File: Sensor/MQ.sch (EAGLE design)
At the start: 4 parts

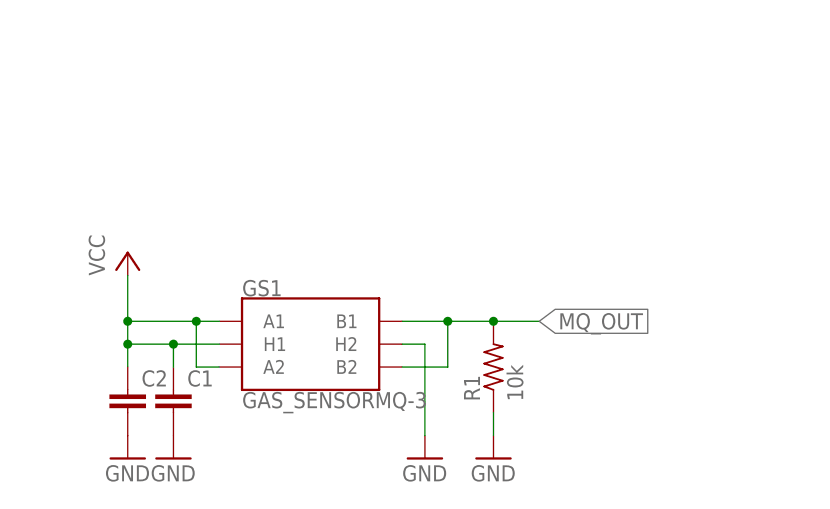
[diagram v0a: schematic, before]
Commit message: Update MQ.sch
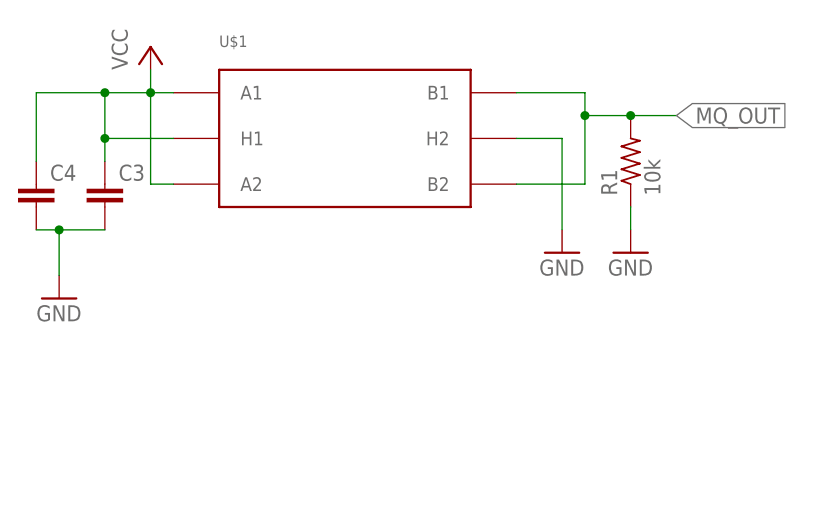
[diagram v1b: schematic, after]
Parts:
- removed C1, C2: (no value), rcl:C-EUC0603
- removed GS1: GAS_SENSORMQ-3, SparkFun-Sensors:GAS_SENSORMQ-3
- added C3, C4: (no value), rcl:C-EUC0603
- added U$1: MQ_GAS_SENSOR_SOCKET, gas_sensor_socket_mq_V2:MQ_GAS_SENSOR_SOCKET
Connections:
- net GND: now also C3.2, C4.2, U$1.H2; no longer C1.2, C2.2, GS1.H2
- net MQ_OUT: now also U$1.B1, U$1.B2; no longer GS1.B1, GS1.B2
- net VCC: now also C3.1, C4.1, U$1.A1, U$1.A2, U$1.H1; no longer C1.1, C2.1, GS1.A1, GS1.A2, GS1.H1
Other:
- moved on the sheet: R1
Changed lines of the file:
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@@
 </classes>
 <parts>
-<part name="P+1" library="supply1" deviceset="VCC" device=""/>
+<part name="U$1" library="gas_sensor_socket_mq_V2" deviceset="MQ_GAS_SENSOR_SOCKET" device=""/>
 <part name="GND1" library="supply1@1" deviceset="GND" device=""/>
 <part name="R1" library="rcl" deviceset="R-US_" device="R0603" value="10k"/>
 <part name="GND2" library="supply1@1" deviceset="GND" device=""/>
-<part name="C1" library="rcl" deviceset="C-EU" device="C0603"/>
-<part name="C2" library="rcl" deviceset="C-EU" device="C0603"/>
-<part name="GND3" library="supply1@1" deviceset="GND" device=""/>
-<part name="GND4" library="supply1@1" deviceset="GND" device=""/>
-<part name="GS1" library="SparkFun-Sensors" deviceset="GAS_SENSOR" device="MQ-3"/>
+<part name="P+2" library="supply1" deviceset="VCC" device=""/>
+<part name="C3" library="rcl" deviceset="C-EU" device="C0603"/>
+<part name="C4" library="rcl" deviceset="C-EU" device="C0603"/>
+<part name="GND5" library="supply1@1" deviceset="GND" device=""/>
 </parts>
 <sheets>
@@
 </plain>
 <instances>
-<instance part="P+1" gate="VCC" x="-5.08" y="88.9" smashed="yes">
-<attribute name="VALUE" x="-7.62" y="86.36" size="1.778" layer="96" rot="R90"/>
+<instance part="U$1" gate="G$1" x="48.26" y="93.98" smashed="yes">
+<attribute name="NAME" x="5.08" y="111.76" size="1.27" layer="95"/>
 </instance>
-<instance part="GND1" gate="1" x="27.94" y="66.04" smashed="yes">
-<attribute name="VALUE" x="25.4" y="63.5" size="1.778" layer="96"/>
+<instance part="GND1" gate="1" x="43.18" y="88.9" smashed="yes">
+<attribute name="VALUE" x="40.64" y="86.36" size="1.778" layer="96"/>
 </instance>
-<instance part="R1" gate="G$1" x="35.56" y="76.2" smashed="yes" rot="R90">
-<attribute name="NAME" x="34.0614" y="72.39" size="1.778" layer="95" rot="R90"/>
-<attribute name="VALUE" x="38.862" y="72.39" size="1.778" layer="96" rot="R90"/>
+<instance part="R1" gate="G$1" x="50.8" y="99.06" smashed="yes" rot="R90">
+<attribute name="NAME" x="49.3014" y="95.25" size="1.778" layer="95" rot="R90"/>
+<attribute name="VALUE" x="54.102" y="95.25" size="1.778" layer="96" rot="R90"/>
 </instance>
-<instance part="GND2" gate="1" x="35.56" y="66.04" smashed="yes">
-<attribute name="VALUE" x="33.02" y="63.5" size="1.778" layer="96"/>
+<instance part="GND2" gate="1" x="50.8" y="88.9" smashed="yes">
+<attribute name="VALUE" x="48.26" y="86.36" size="1.778" layer="96"/>
 </instance>
-<instance part="C1" gate="G$1" x="0" y="73.66" smashed="yes">
-<attribute name="NAME" x="1.524" y="74.041" size="1.778" layer="95"/>
-<attribute name="VALUE" x="1.524" y="68.961" size="1.778" layer="96"/>
+<instance part="P+2" gate="VCC" x="-2.54" y="111.76" smashed="yes">
+<attribute name="VALUE" x="-5.08" y="109.22" size="1.778" layer="96" rot="R90"/>
 </instance>
-<instance part="C2" gate="G$1" x="-5.08" y="73.66" smashed="yes">
-<attribute name="NAME" x="-3.556" y="74.041" size="1.778" layer="95"/>
-<attribute name="VALUE" x="-3.556" y="68.961" size="1.778" layer="96"/>
+<instance part="C3" gate="G$1" x="-7.62" y="96.52" smashed="yes">
+<attribute name="NAME" x="-6.096" y="96.901" size="1.778" layer="95"/>
+<attribute name="VALUE" x="-6.096" y="91.821" size="1.778" layer="96"/>
 </instance>
-<instance part="GND3" gate="1" x="-5.08" y="66.04" smashed="yes">
-<attribute name="VALUE" x="-7.62" y="63.5" size="1.778" layer="96"/>
+<instance part="C4" gate="G$1" x="-15.24" y="96.52" smashed="yes">
+<attribute name="NAME" x="-13.716" y="96.901" size="1.778" layer="95"/>
+<attribute name="VALUE" x="-13.716" y="91.821" size="1.778" layer="96"/>
 </instance>
-<instance part="GND4" gate="1" x="0" y="66.04" smashed="yes">
-<attribute name="VALUE" x="-2.54" y="63.5" size="1.778" layer="96"/>
-</instance>
-<instance part="GS1" gate="G$1" x="15.24" y="78.74" smashed="yes">
-<attribute name="NAME" x="7.62" y="84.074" size="1.778" layer="95" font="vector"/>
-<attribute name="VALUE" x="7.62" y="73.406" size="1.778" layer="96" font="vector" align="top-left"/>
+<instance part="GND5" gate="1" x="-12.7" y="83.82" smashed="yes">
+<attribute name="VALUE" x="-15.24" y="81.28" size="1.778" layer="96"/>
 </instance>
 </instances>
@@
 <net name="VCC" class="0">
 <segment>
-<wire x1="5.08" y1="78.74" x2="0" y2="78.74" width="0.1524" layer="91"/>
-<wire x1="0" y1="78.74" x2="-5.08" y2="78.74" width="0.1524" layer="91"/>
-<wire x1="-5.08" y1="78.74" x2="-5.08" y2="81.28" width="0.1524" layer="91"/>
-<wire x1="-5.08" y1="81.28" x2="2.54" y2="81.28" width="0.1524" layer="91"/>
-<pinref part="P+1" gate="VCC" pin="VCC"/>
-<wire x1="2.54" y1="81.28" x2="5.08" y2="81.28" width="0.1524" layer="91"/>
-<wire x1="-5.08" y1="86.36" x2="-5.08" y2="81.28" width="0.1524" layer="91"/>
-<junction x="-5.08" y="81.28"/>
-<pinref part="C2" gate="G$1" pin="1"/>
-<wire x1="-5.08" y1="76.2" x2="-5.08" y2="78.74" width="0.1524" layer="91"/>
-<junction x="-5.08" y="78.74"/>
-<pinref part="C1" gate="G$1" pin="1"/>
-<wire x1="0" y1="76.2" x2="0" y2="78.74" width="0.1524" layer="91"/>
-<junction x="0" y="78.74"/>
-<pinref part="GS1" gate="G$1" pin="A1"/>
-<pinref part="GS1" gate="G$1" pin="H1"/>
-<pinref part="GS1" gate="G$1" pin="A2"/>
-<wire x1="5.08" y1="76.2" x2="2.54" y2="76.2" width="0.1524" layer="91"/>
-<wire x1="2.54" y1="76.2" x2="2.54" y2="81.28" width="0.1524" layer="91"/>
-<junction x="2.54" y="81.28"/>
+<pinref part="U$1" gate="G$1" pin="A2"/>
+<wire x1="0" y1="96.52" x2="-2.54" y2="96.52" width="0.1524" layer="91"/>
+<wire x1="-2.54" y1="96.52" x2="-2.54" y2="106.68" width="0.1524" layer="91"/>
+<pinref part="U$1" gate="G$1" pin="A1"/>
+<wire x1="-2.54" y1="106.68" x2="0" y2="106.68" width="0.1524" layer="91"/>
+<pinref part="P+2" gate="VCC" pin="VCC"/>
+<wire x1="-2.54" y1="109.22" x2="-2.54" y2="106.68" width="0.1524" layer="91"/>
+<junction x="-2.54" y="106.68"/>
+<wire x1="-2.54" y1="106.68" x2="-7.62" y2="106.68" width="0.1524" layer="91"/>
+<pinref part="C4" gate="G$1" pin="1"/>
+<wire x1="-7.62" y1="106.68" x2="-15.24" y2="106.68" width="0.1524" layer="91"/>
+<wire x1="-15.24" y1="106.68" x2="-15.24" y2="99.06" width="0.1524" layer="91"/>
+<pinref part="C3" gate="G$1" pin="1"/>
+<wire x1="-7.62" y1="99.06" x2="-7.62" y2="101.6" width="0.1524" layer="91"/>
+<junction x="-7.62" y="106.68"/>
+<pinref part="U$1" gate="G$1" pin="H1"/>
+<wire x1="-7.62" y1="101.6" x2="-7.62" y2="106.68" width="0.1524" layer="91"/>
+<wire x1="0" y1="101.6" x2="-7.62" y2="101.6" width="0.1524" layer="91"/>
+<junction x="-7.62" y="101.6"/>
 </segment>
 </net>
 <net name="GND" class="0">
 <segment>
+<wire x1="43.18" y1="91.44" x2="43.18" y2="101.6" width="0.1524" layer="91"/>
 <pinref part="GND1" gate="1" pin="GND"/>
-<wire x1="27.94" y1="68.58" x2="27.94" y2="78.74" width="0.1524" layer="91"/>
-<wire x1="27.94" y1="78.74" x2="25.4" y2="78.74" width="0.1524" layer="91"/>
-<pinref part="GS1" gate="G$1" pin="H2"/>
+<pinref part="U$1" gate="G$1" pin="H2"/>
+<wire x1="38.1" y1="101.6" x2="43.18" y2="101.6" width="0.1524" layer="91"/>
 </segment>
 <segment>
+<wire x1="50.8" y1="93.98" x2="50.8" y2="91.44" width="0.1524" layer="91"/>
 <pinref part="R1" gate="G$1" pin="1"/>
 <pinref part="GND2" gate="1" pin="GND"/>
-<wire x1="35.56" y1="71.12" x2="35.56" y2="68.58" width="0.1524" layer="91"/>
 </segment>
 <segment>
-<pinref part="C2" gate="G$1" pin="2"/>
-<pinref part="GND3" gate="1" pin="GND"/>
-</segment>
-<segment>
-<pinref part="C1" gate="G$1" pin="2"/>
-<pinref part="GND4" gate="1" pin="GND"/>
+<pinref part="C3" gate="G$1" pin="2"/>
+<pinref part="C4" gate="G$1" pin="2"/>
+<wire x1="-7.62" y1="91.44" x2="-12.7" y2="91.44" width="0.1524" layer="91"/>
+<pinref part="GND5" gate="1" pin="GND"/>
+<wire x1="-12.7" y1="91.44" x2="-15.24" y2="91.44" width="0.1524" layer="91"/>
+<wire x1="-12.7" y1="86.36" x2="-12.7" y2="91.44" width="0.1524" layer="91"/>
+<junction x="-12.7" y="91.44"/>
 </segment>
 </net>
 <net name="MQ_OUT" class="0">
 <segment>
+<wire x1="45.72" y1="104.14" x2="50.8" y2="104.14" width="0.1524" layer="91"/>
+<wire x1="50.8" y1="104.14" x2="55.88" y2="104.14" width="0.1524" layer="91"/>
+<junction x="50.8" y="104.14"/>
+<label x="55.88" y="104.14" size="1.778" layer="95" xref="yes"/>
+<wire x1="45.72" y1="96.52" x2="45.72" y2="104.14" width="0.1524" layer="91"/>
+<junction x="45.72" y="104.14"/>
 <pinref part="R1" gate="G$1" pin="2"/>
-<wire x1="25.4" y1="81.28" x2="30.48" y2="81.28" width="0.1524" layer="91"/>
-<wire x1="30.48" y1="81.28" x2="35.56" y2="81.28" width="0.1524" layer="91"/>
-<wire x1="35.56" y1="81.28" x2="40.64" y2="81.28" width="0.1524" layer="91"/>
-<junction x="35.56" y="81.28"/>
-<label x="40.64" y="81.28" size="1.778" layer="95" xref="yes"/>
-<pinref part="GS1" gate="G$1" pin="B1"/>
-<pinref part="GS1" gate="G$1" pin="B2"/>
-<wire x1="25.4" y1="76.2" x2="30.48" y2="76.2" width="0.1524" layer="91"/>
-<wire x1="30.48" y1="76.2" x2="30.48" y2="81.28" width="0.1524" layer="91"/>
-<junction x="30.48" y="81.28"/>
+<pinref part="U$1" gate="G$1" pin="B1"/>
+<wire x1="38.1" y1="106.68" x2="45.72" y2="106.68" width="0.1524" layer="91"/>
+<wire x1="45.72" y1="106.68" x2="45.72" y2="104.14" width="0.1524" layer="91"/>
+<pinref part="U$1" gate="G$1" pin="B2"/>
+<wire x1="38.1" y1="96.52" x2="45.72" y2="96.52" width="0.1524" layer="91"/>
 </segment>
 </net>
